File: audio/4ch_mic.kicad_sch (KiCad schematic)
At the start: 41 parts, among them U10 ac108, U11 TCR3RM33, U12 TCR3RM33, U15 MIC_4PIN_SMD, U16 MIC_4PIN_SMD, U17 MIC_4PIN_SMD, U18 MIC_4PIN_SMD, X1 ASE-24.000MHz

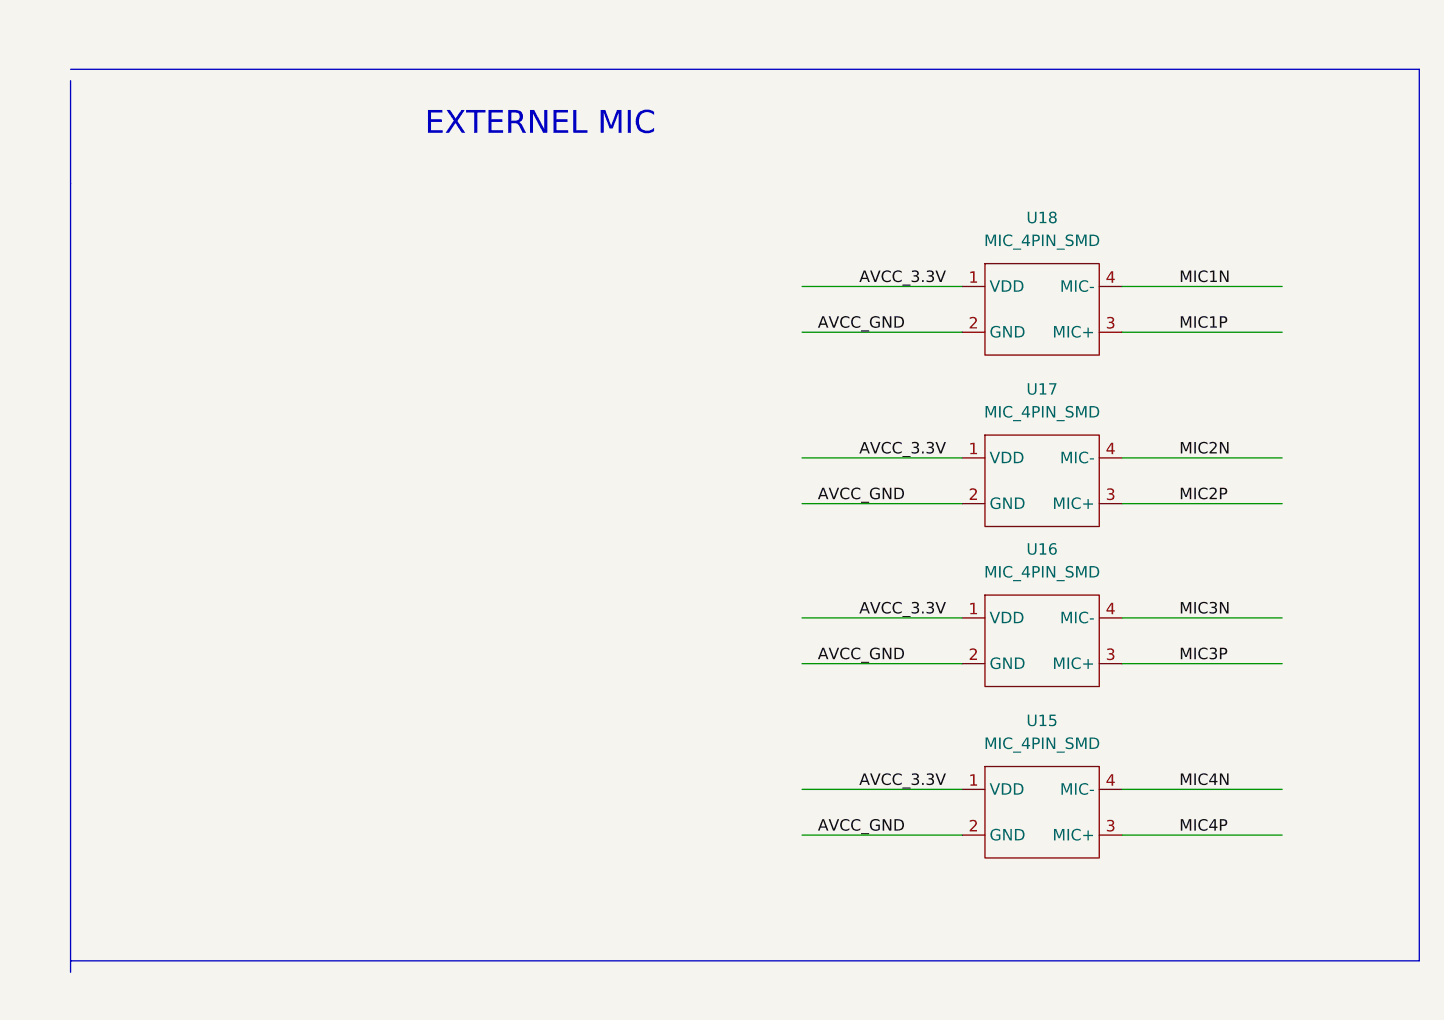
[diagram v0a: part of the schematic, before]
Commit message: .
.
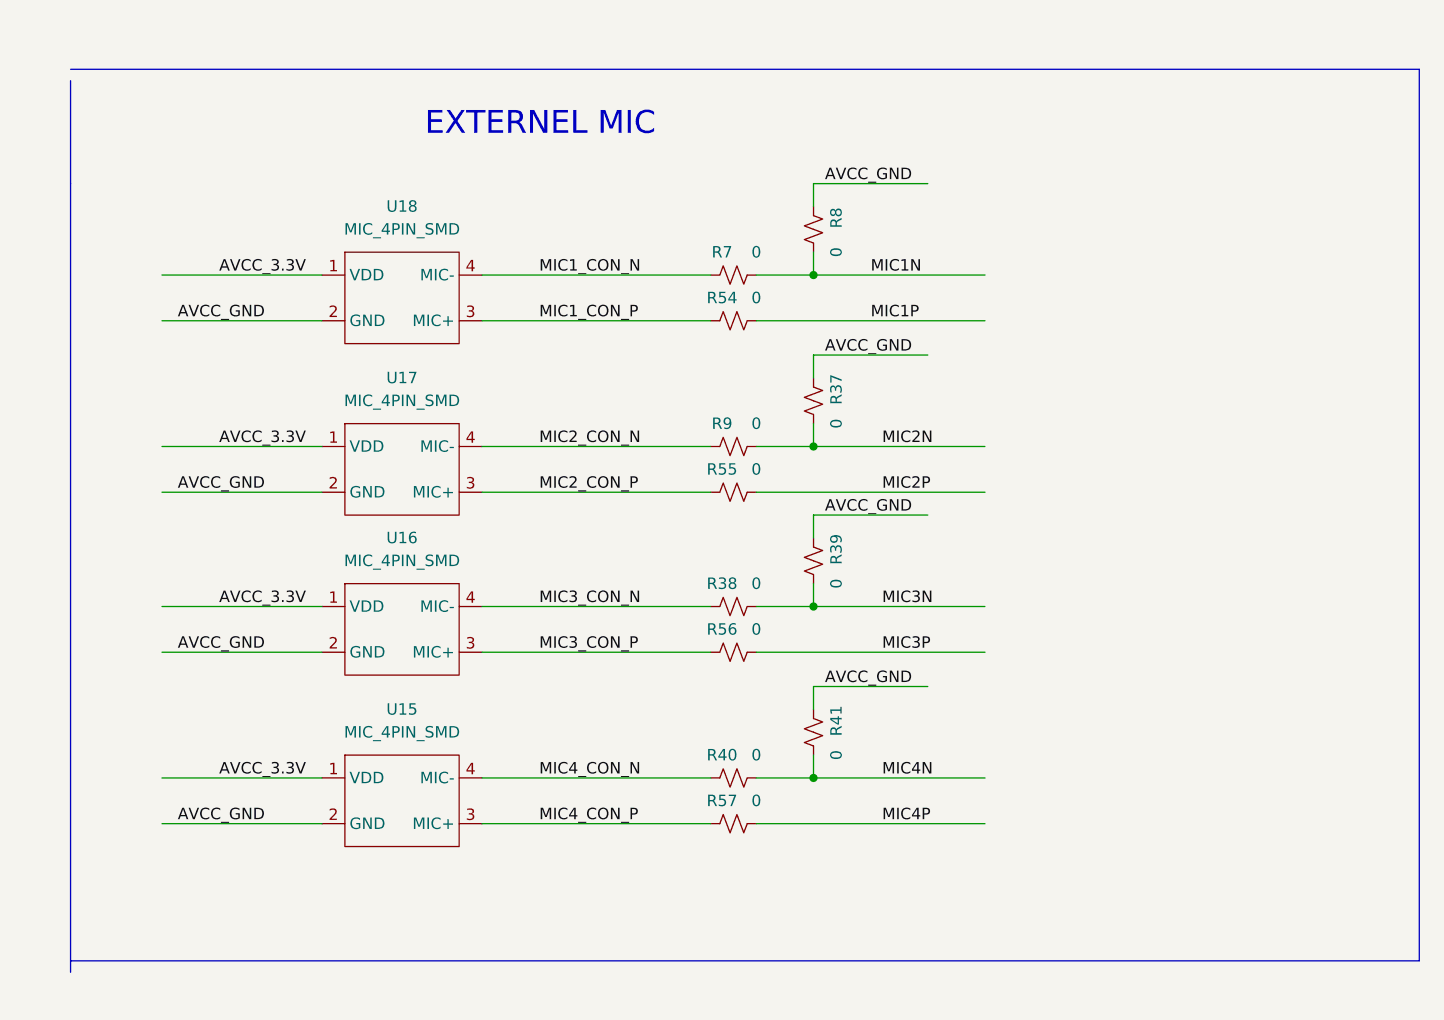
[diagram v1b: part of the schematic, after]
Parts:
- added R37, R38, R39, R40, R41, R54, R55, R56, R57, R7, R8, R9: 0, Resistor_SMD:R_0402_1005Metric, symbol Device:R_Small_US
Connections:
- net AVCC_GND: now also R37.1, R39.1, R41.1, R8.1
- net MIC1N: now also R7.2, R8.2; no longer U18.4 (MIC-)
- net MIC1P: now also R54.2; no longer U18.3 (MIC+)
- net MIC2N: now also R37.2, R9.2; no longer U17.4 (MIC-)
- net MIC2P: now also R55.2; no longer U17.3 (MIC+)
- net MIC3N: now also R38.2, R39.2; no longer U16.4 (MIC-)
- net MIC3P: now also R56.2; no longer U16.3 (MIC+)
- net MIC4N: now also R40.2, R41.2; no longer U15.4 (MIC-)
- net MIC4P: now also R57.2; no longer U15.3 (MIC+)
- new net MIC1_CON_N: R7.1, U18.4 (MIC-)
- new net MIC1_CON_P: R54.1, U18.3 (MIC+)
- new net MIC2_CON_N: R9.1, U17.4 (MIC-)
- new net MIC2_CON_P: R55.1, U17.3 (MIC+)
- new net MIC3_CON_N: R38.1, U16.4 (MIC-)
- new net MIC3_CON_P: R56.1, U16.3 (MIC+)
- new net MIC4_CON_N: R40.1, U15.4 (MIC-)
- new net MIC4_CON_P: R57.1, U15.3 (MIC+)
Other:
- moved on the sheet: U15, U16, U17, U18
